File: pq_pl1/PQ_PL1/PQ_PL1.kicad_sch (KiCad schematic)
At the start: 5 parts, among them J1 Conn_01x10, J2 Conn_01x10, J3 Conn_01x10, J4 Conn_01x10, J5 Conn_01x04

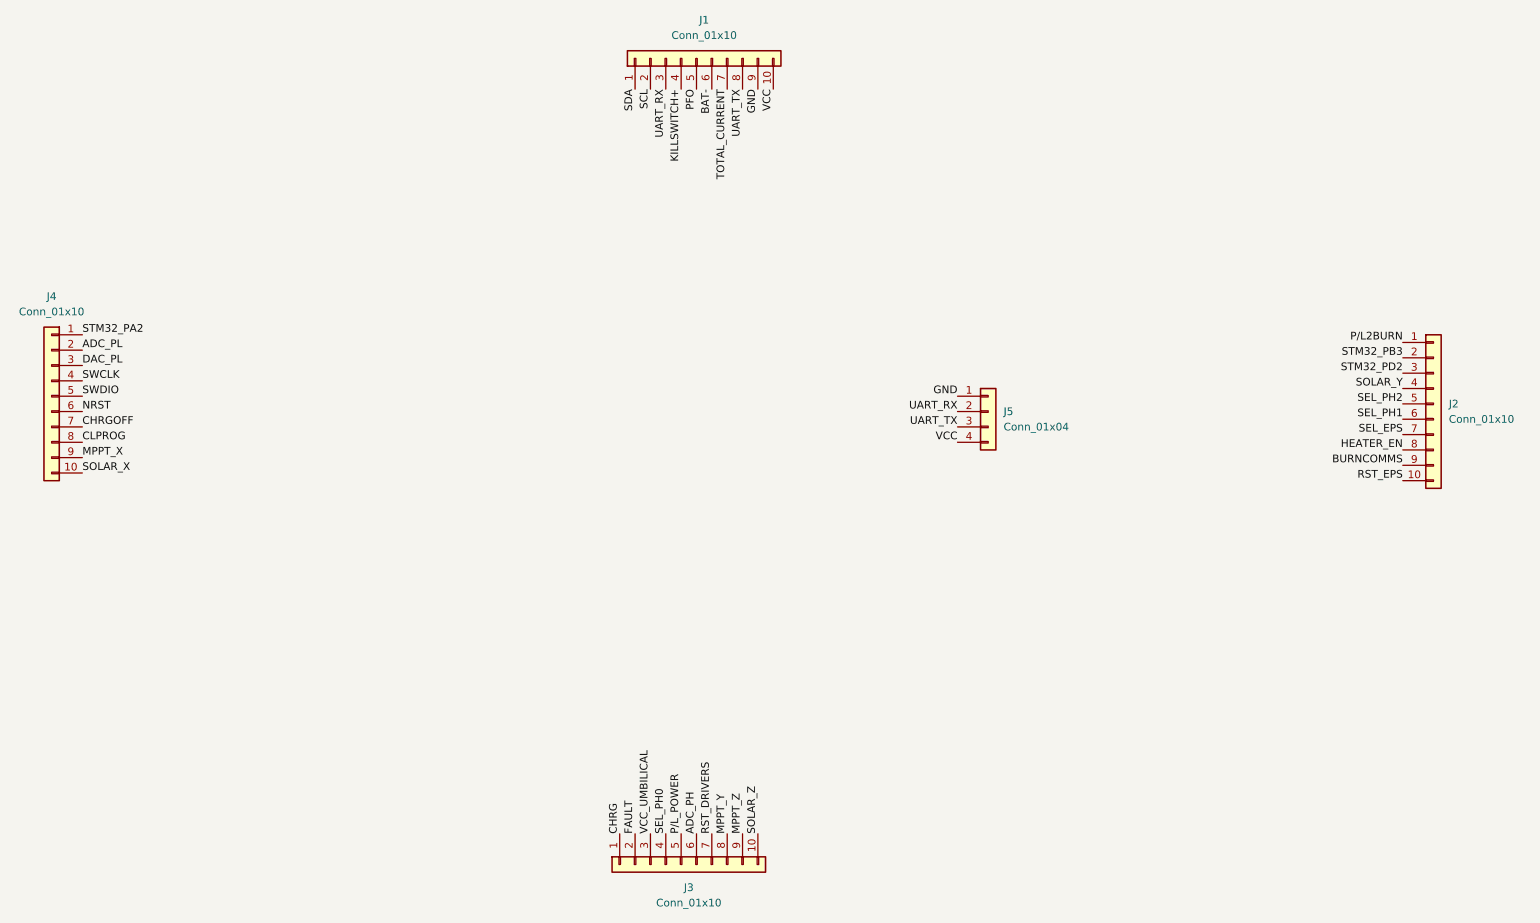
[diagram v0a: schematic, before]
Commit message: Functional revision and finishing touches part II
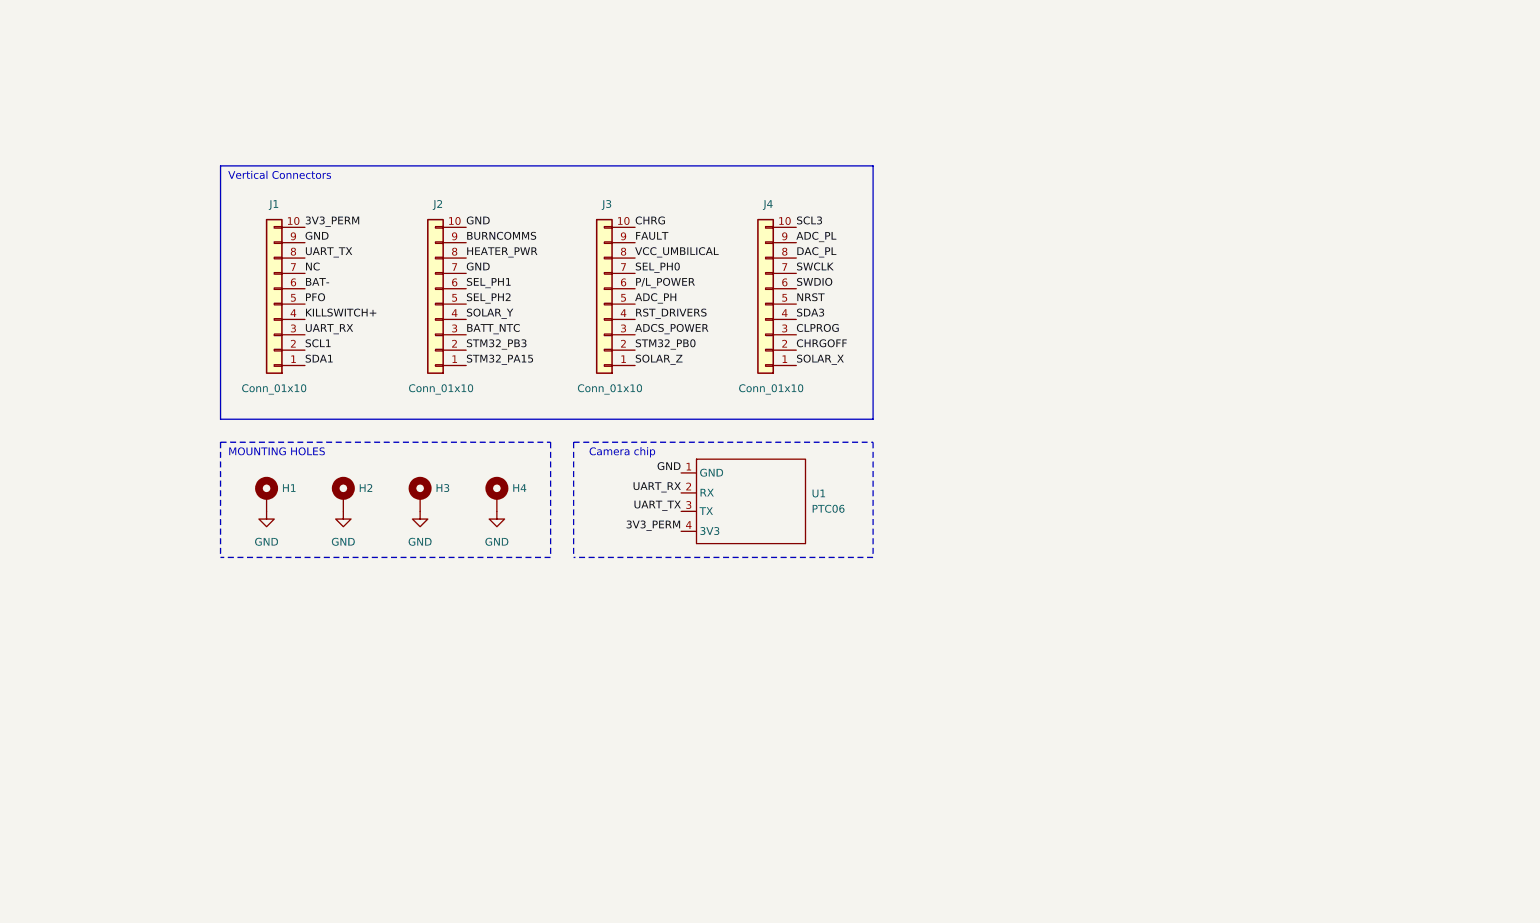
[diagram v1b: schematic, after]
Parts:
- removed J5: Conn_01x04, Connector_PinSocket_2.00mm:PinSocket_1x04_P2.00mm_Vertical, symbol Connector_Generic:Conn_01x04
- added H1, H2, H3, H4: MountingHole_Pad, MountingHole:MountingHole_3.2mm_M3_Pad, symbol Mechanical:MountingHole_Pad
- added U1: PTC06, sensor-nsl:PTC06, symbol sensor-nsl:PTC06
- J1: footprint Connector_PinSocket_2.54mm:PinSocket_1x10_P2.54mm_Vertical -> connector-nsl:SLW-110-01
- J2, J3, J4: footprint (none) -> connector-nsl:SLW-110-01
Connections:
- net MPPT_X is gone; now on net ADC_PL: J4.9 (Pin_9)
- net MPPT_Y is gone; now on net VCC_UMBILICAL: J3.8 (Pin_8)
- net MPPT_Z is gone; now on net FAULT: J3.9 (Pin_9)
- net RST_EPS is gone; now on net GND: J2.10 (Pin_10)
- net SEL_EPS is gone; now on net GND: J2.7 (Pin_7)
- net STM32_PA2 is gone; now on net SOLAR_X: J4.1 (Pin_1)
- net ADC_PH: now also J3.5 (Pin_5); no longer J3.6 (Pin_6)
- net ADC_PL: no longer J4.2 (Pin_2)
- net CHRG: now also J3.10 (Pin_10); no longer J3.1 (Pin_1)
- net CHRGOFF: now also J4.2 (Pin_2); no longer J4.7 (Pin_7)
- net CLPROG: now also J4.3 (Pin_3); no longer J4.8 (Pin_8)
- net DAC_PL: now also J4.8 (Pin_8); no longer J4.3 (Pin_3)
- net FAULT: no longer J3.2 (Pin_2)
- net GND: now also H1.1, H2.1, H3.1, H4.1, U1.1 (GND)
- net NRST: now also J4.5 (Pin_5); no longer J4.6 (Pin_6)
- net P/L_POWER: now also J3.6 (Pin_6); no longer J3.5 (Pin_5)
- net RST_DRIVERS: now also J3.4 (Pin_4); no longer J3.7 (Pin_7)
- net SEL_PH0: now also J3.7 (Pin_7); no longer J3.4 (Pin_4)
- net SOLAR_X: no longer J4.10 (Pin_10)
- net SOLAR_Z: now also J3.1 (Pin_1); no longer J3.10 (Pin_10)
- net SWCLK: now also J4.7 (Pin_7); no longer J4.4 (Pin_4)
- net SWDIO: now also J4.6 (Pin_6); no longer J4.5 (Pin_5)
- net UART_RX: now also U1.2 (RX)
- net UART_TX: now also U1.3 (TX)
- net VCC_UMBILICAL: no longer J3.3 (Pin_3)
- net HEATER_EN renamed HEATER_PWR
- net P/L2BURN renamed STM32_PA15
- net SCL renamed SCL1
- net SDA renamed SDA1
- net STM32_PD2 renamed BATT_NTC
- net TOTAL_CURRENT renamed NC
- net VCC renamed 3V3_PERM
- net 3V3_PERM: now also U1.4 (3V3)
- new net ADCS_POWER: J3.3 (Pin_3)
- new net SCL3: J4.10 (Pin_10)
- new net SDA3: J4.4 (Pin_4)
- new net STM32_PB0: J3.2 (Pin_2)
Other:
- note added: "Camera chip"
- note added: "MOUNTING HOLES"
- note added: "Vertical Connectors"
- moved on the sheet: J1, J2
